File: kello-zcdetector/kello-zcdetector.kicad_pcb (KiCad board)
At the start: 2 copper layers, 10 parts, among them J1 Conn_01x02_Male, J2 Conn_01x02_Male, U1 LTV-817S

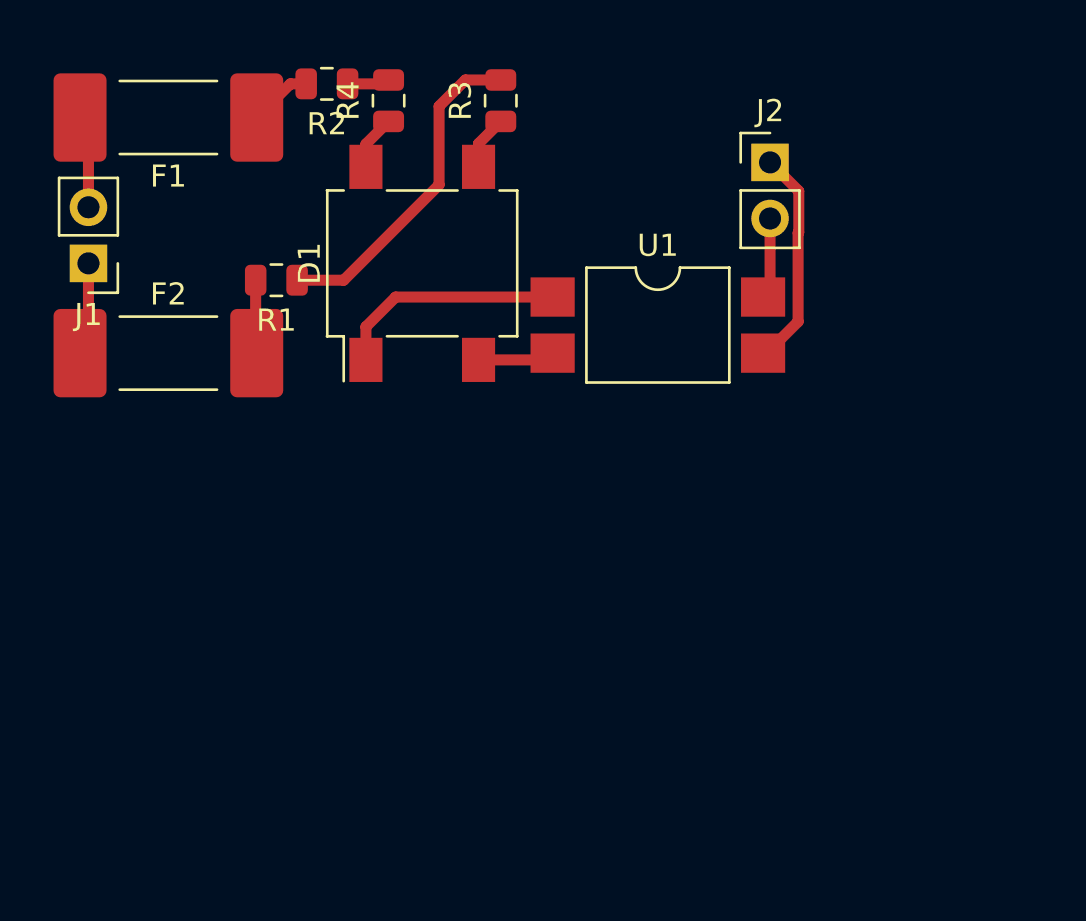
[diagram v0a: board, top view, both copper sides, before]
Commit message: jawohl
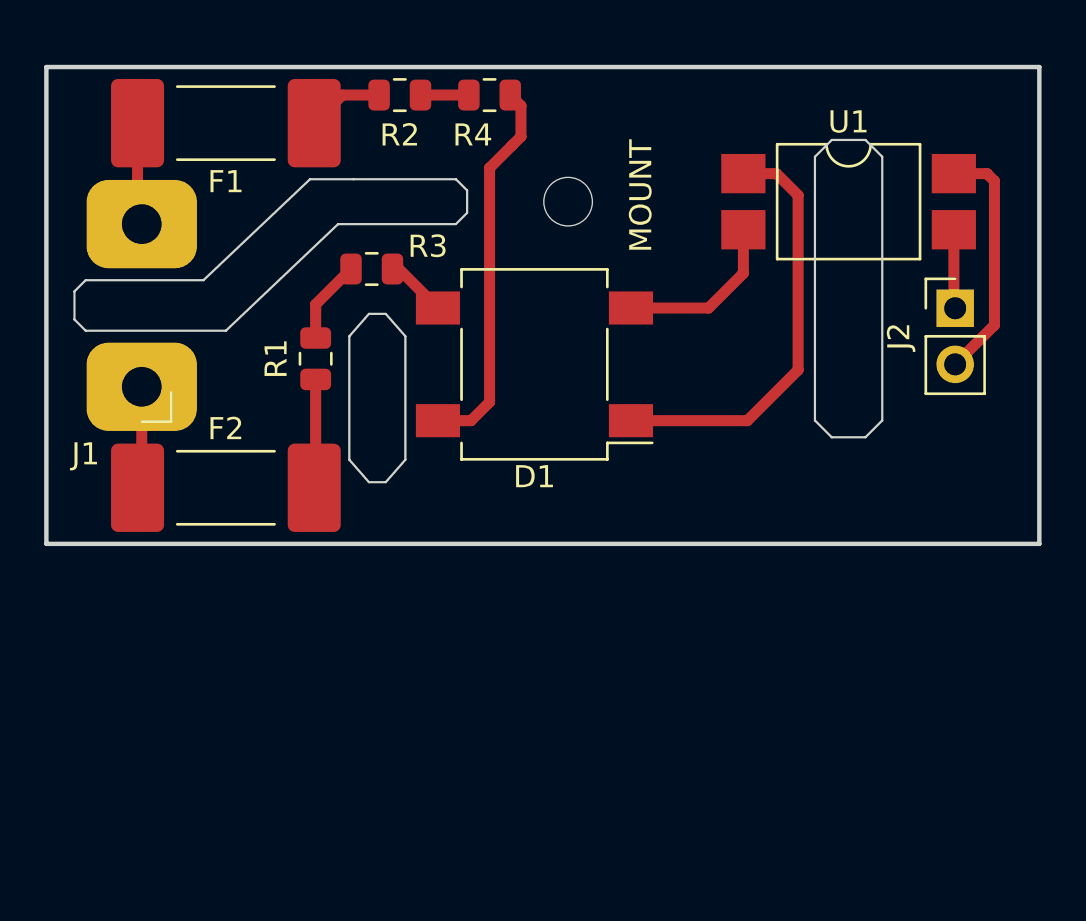
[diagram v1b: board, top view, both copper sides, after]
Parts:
- added MOUNT: MountingHole_2.2mm_M2, MountingHole:MountingHole_2.2mm_M2, F.Cu at (35.7, 18.2)
- J1: footprint Connector_PinHeader_2.54mm:PinHeader_1x02_P2.54mm_Vertical -> Connector_PinHeader_2.54mm:AC_connector
- moved J2 10.7 mm to (53.2, 23.0)
- moved U1 10.3 mm to (48.4, 18.2)
- moved R3 9.60 mm to (26.8, 21.2), turned to 180 degrees
- moved D1 6.83 mm to (34.2, 25.5), turned to 180 degrees
- moved F2 6.63 mm to (20.2, 31.1)
- moved J1 6.32 mm to (16.4, 26.8)
- moved R4 4.58 mm to (32.1, 13.3), turned to 180 degrees
- moved R1 3.98 mm to (24.3, 25.3), turned to 270 degrees
- moved R2 3.34 mm to (28.1, 13.3)
- moved F1 2.62 mm to (20.2, 14.6)
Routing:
- net Net-(D1-Pad4): track 2.48 -> 17.4 mm
- net Net-(R1-Pad1): track 15.1 -> 3.79 mm
- net Net-(D1-Pad1): track 10.5 -> 19.3 mm
- net Net-(J2-Pad2): track 3.69 -> 11.0 mm
- net Net-(J2-Pad1): track 9.94 -> 3.58 mm
- net Net-(D1-Pad2): track 3.48 -> 7.71 mm
- net Net-(F2-Pad2): track 3.32 -> 5.20 mm
- net Net-(F2-Pad1): track 4.14 -> 5.91 mm
- net Net-(F1-Pad1): track 2.87 -> 3.46 mm
- net Net-(F1-Pad2): track 4.14 -> 4.65 mm
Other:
- board outline added: 45 x 21.6 mm

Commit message: joo
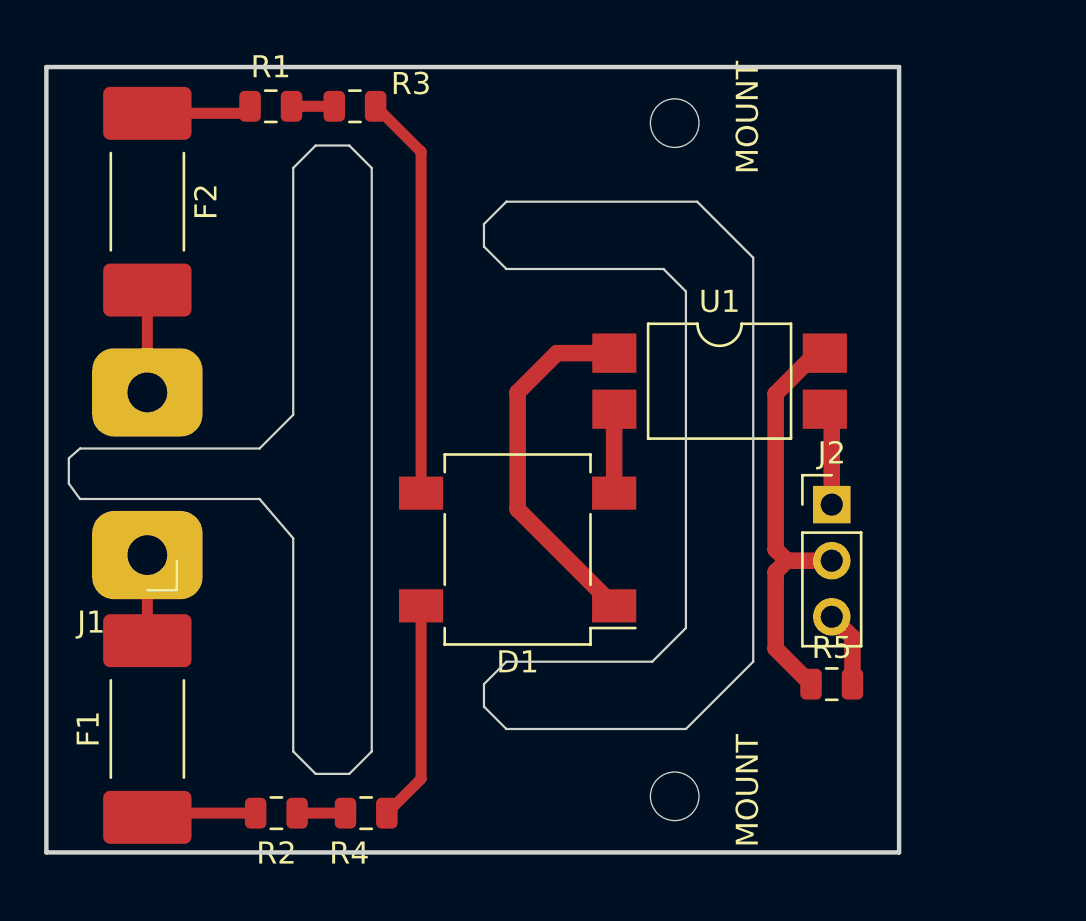
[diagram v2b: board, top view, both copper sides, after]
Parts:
- removed the MOUNT at (35.7, 18.2)
- added MOUNT: MountingHole_2.2mm_M2, MountingHole:MountingHole_2.2mm_M2, F.Cu at (40.5, 45.1)
- added MOUNT: MountingHole_2.2mm_M2, MountingHole:MountingHole_2.2mm_M2, F.Cu at (40.5, 14.6)
- added R5: 47k, Resistor_SMD:R_0805_2012Metric, F.Cu at (47.6, 40.0)
- J2: footprint Connector_PinHeader_2.54mm:PinHeader_1x02_P2.54mm_Vertical -> Connector_PinHeader_2.54mm:PinHeader_1x03_P2.54mm_Vertical
- moved R2 33.0 mm to (22.5, 45.8)
- moved R4 33.0 mm to (26.5, 45.8)
- moved F1 27.7 mm to (16.6, 42.0), turned to 90 degrees
- moved F2 13.4 mm to (16.6, 18.2), turned to 270 degrees
- moved R1 11.6 mm to (22.2, 13.8), turned to 180 degrees
- moved J2 10.5 mm to (47.6, 31.9)
- moved U1 10.0 mm to (42.5, 26.3)
- moved D1 8.42 mm to (33.4, 33.9)
- moved J1 7.62 mm to (16.6, 34.4)
- moved R3 7.41 mm to (26.0, 13.8)
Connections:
- J1 pad 1: Net-(F2-Pad1) -> Net-(F1-Pad2)
- J1 pad 2: Net-(F1-Pad2) -> Net-(F2-Pad2)
- R1 pad 2: Net-(F2-Pad2) -> Net-(F2-Pad1)
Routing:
- net Net-(D1-Pad3): track 2.79 -> 18.4 mm
- net Net-(J2-Pad2): track 11.0 -> 19.2 mm
- net Net-(D1-Pad4): track 17.4 -> 10.0 mm
- net Net-(D1-Pad2): track 7.71 -> 3.80 mm
- net Net-(J2-Pad3): track 0.00 -> 3.44 mm
- net Net-(D1-Pad1): track 19.3 -> 16.6 mm
- net Net-(R1-Pad1): track 3.79 -> 1.93 mm
- net Net-(F1-Pad1): track 3.46 -> 4.98 mm
- net Net-(F2-Pad1): track 5.91 -> 4.78 mm
- net Net-(J2-Pad1): track 3.58 -> 4.45 mm
- net Net-(F2-Pad2): track 5.20 -> 4.64 mm
- net Net-(F1-Pad2): track 4.65 -> 4.14 mm
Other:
- board size 45 x 21.6 mm -> 38.6 x 35.6 mm
